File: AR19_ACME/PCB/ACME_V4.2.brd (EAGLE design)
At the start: 47 x 34.1 mm, 23 parts, among them IC1 Optocoupler DIP, Q1 NGD8201ANT4G, Q2 NGD8201ANT4G

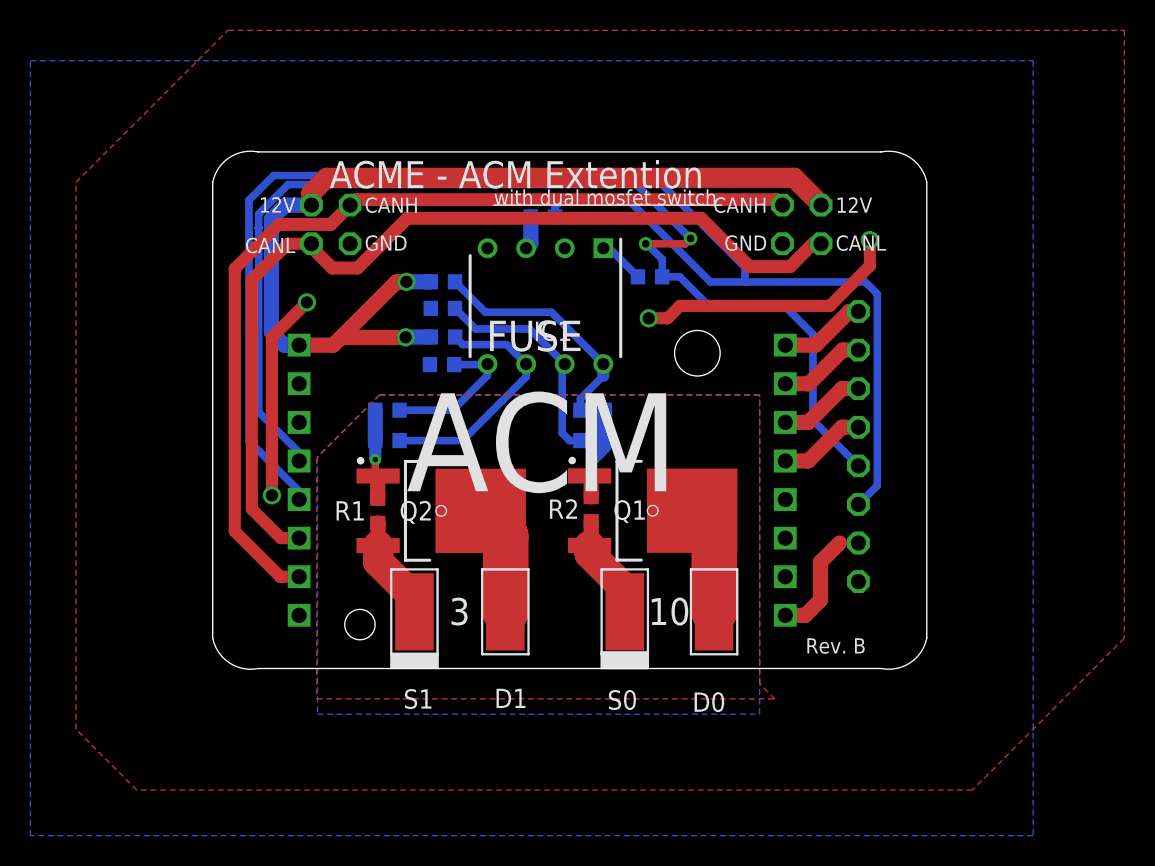
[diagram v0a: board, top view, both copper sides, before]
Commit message: ACME V4.2
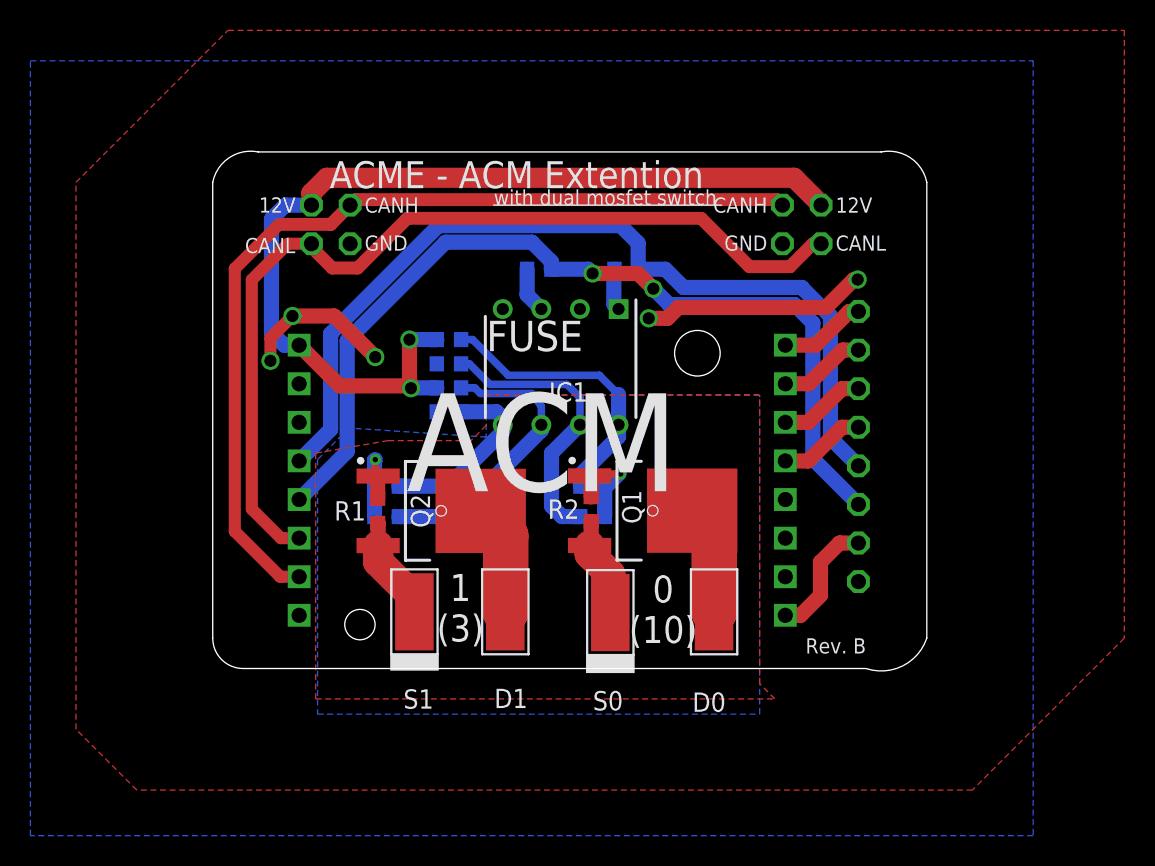
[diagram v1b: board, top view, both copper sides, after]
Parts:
- moved N_FET11 5.00 mm to (12.4, 12.0)
- moved P_FET1 5.00 mm to (12.4, 10.0)
- moved N_FET10 5.00 mm to (26.0, 10.0)
- moved P_FET0 5.00 mm to (26.0, 12.0)
- moved IC1 4.12 mm to (23.9, 19.9)
- moved N_FET0 3.82 mm to (16.6, 21.6)
- moved P_FET10 3.67 mm to (16.6, 20.1)
- moved R4 3.45 mm to (22.5, 26.3)
- moved N_FET1 3.37 mm to (16.6, 18.5)
- moved P_FET11 3.13 mm to (16.6, 16.9)
- moved R3 1.63 mm to (28.2, 26.3)
- moved S0 0.95 mm to (27.2, 3.68)
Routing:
- net PWM1: track 96.9 -> 60.8 mm, vias 0 -> 2
- net PWM0: track 75.2 -> 59.1 mm, vias 2 -> 0
- net GND: track 31.3 -> 24.9 mm, vias 4 -> 5
- net N$9: track 14.8 -> 18.8 mm
- net N$4: track 15.7 -> 18.9 mm
- net N$5: track 16.3 -> 19.2 mm
- net GATE0: track 6.16 -> 8.76 mm
- net N$8: track 9.70 -> 12.1 mm
- net 5V: track 7.01 -> 8.06 mm
- net 12V: track 64.5 -> 63.4 mm
- net N$6: track 2.19 -> 3.01 mm
- net GATE1: track 5.91 -> 6.43 mm
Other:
- board size 47 x 34.1 mm -> 47 x 34.2 mm
- board text added: "0 (10)"
- board text added: "1 (3)"
- board text added: "White pad: N-Mosfet: GND P-Mosfet: 12V"
- board text added: "v4.2"
- board text removed: "10"
- board text removed: "3"
- board text removed: "N-Mosfet - ■ GND P-Mosfet - ■ 12V ■ Pull up or pull down"
- board text removed: "v4.1"
